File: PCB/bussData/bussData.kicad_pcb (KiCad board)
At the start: 2 copper layers, 104.1 x 57.2 mm, 13 parts, among them M3 MountingHole_3.2mm_M3

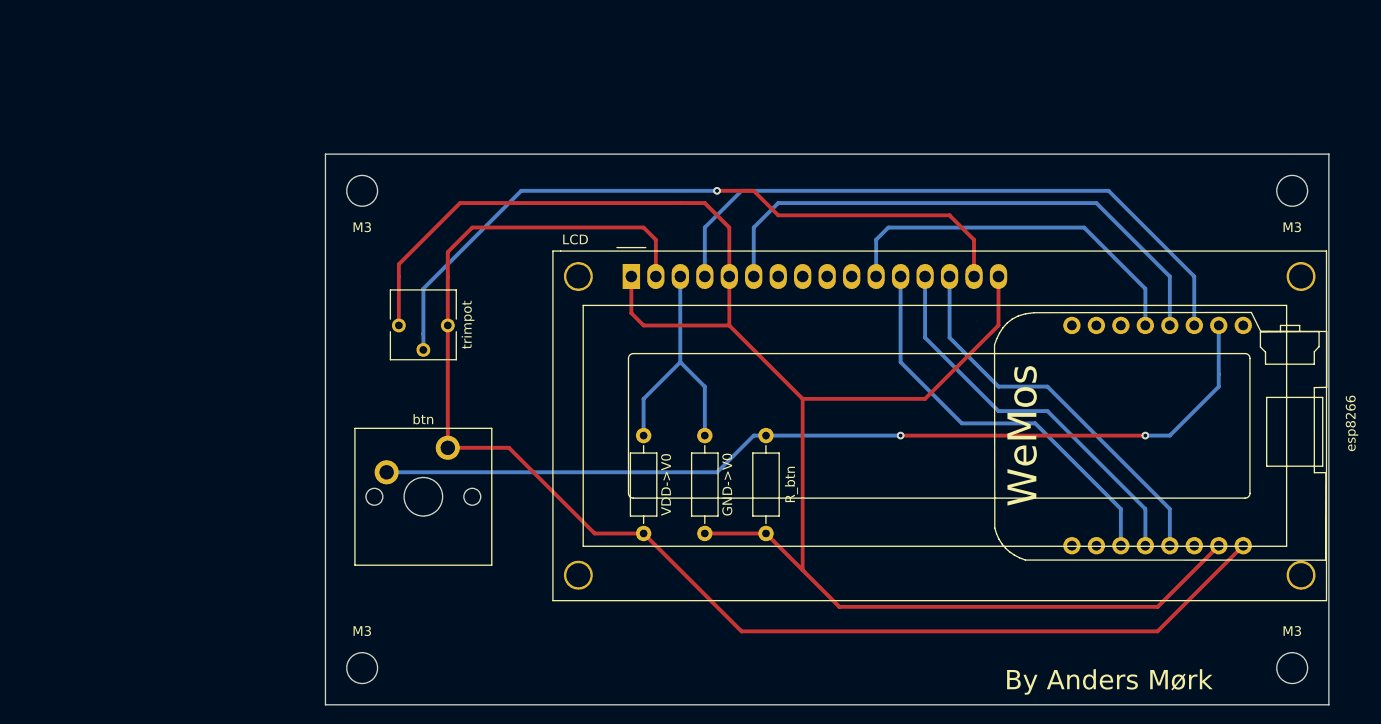
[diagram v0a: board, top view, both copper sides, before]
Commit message: updated pcb
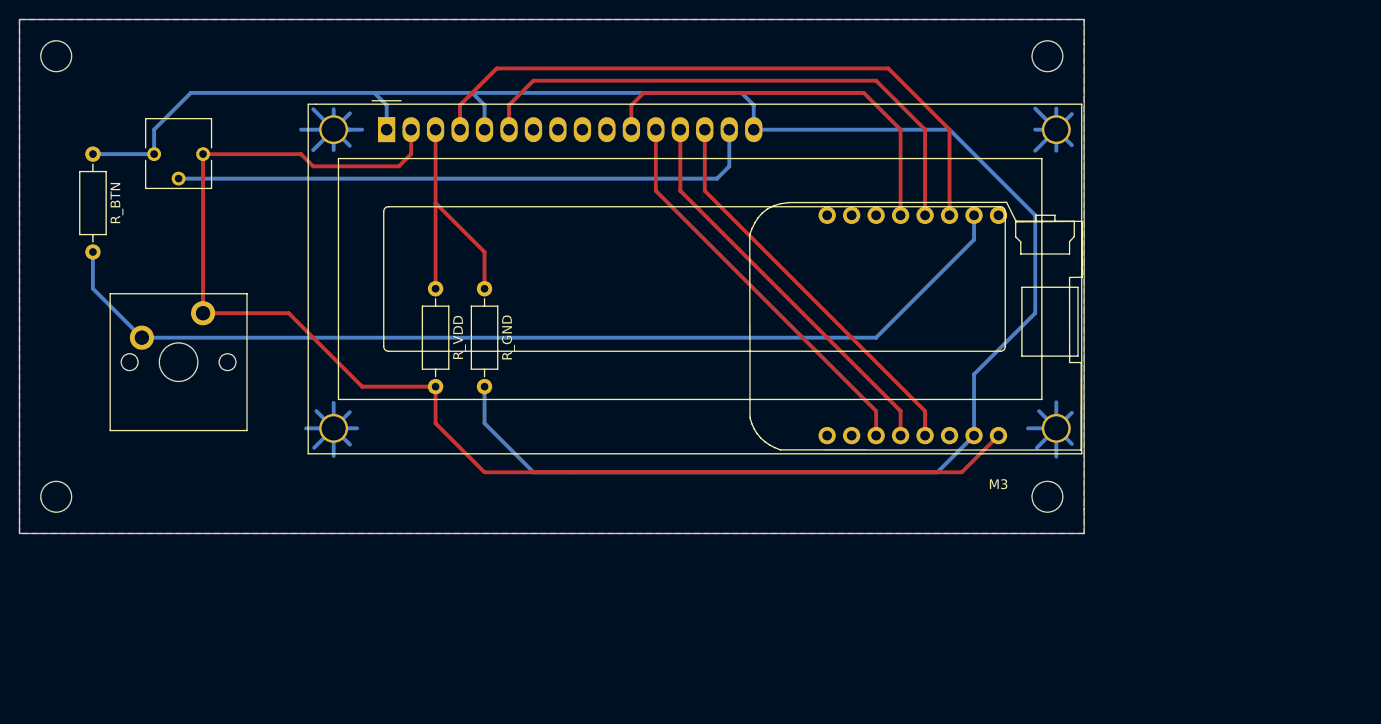
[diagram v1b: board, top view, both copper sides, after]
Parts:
- removed ? (x2): , 
- removed GND->V0, R_btn, VDD->V0: ?, Resistor_THT:R_Axial_DIN0207_L6.3mm_D2.5mm_P10.16mm_Horizontal
- removed LCD: RC1602A, Display:WC1602A
- removed the M3 at (209.6, 72.4)
- removed the M3 at (209.6, 121.9)
- removed the M3 at (113.0, 72.4)
- removed the M3 at (113.0, 121.9)
- removed btn: SW_Push_Open, Switch_Keyboard_Cherry_MX:SW_Cherry_MX_PCB_1.00u
- removed esp8266: WeMos_d1_mini, Module:D1_mini_board
- removed trimpot: R_POT_TRIM, Potentiometer_THT:Potentiometer_Vishay_T73YP_Vertical
- added DIM1: R_POT_TRIM, Potentiometer_THT:Potentiometer_Vishay_T73YP_Vertical, F.Cu at (91.4, 68.6)
- added LCD1: RC1602A, Display:WC1602A, F.Cu at (115.6, 66.0)
- added M3: MountingHole_3.2mm_M3, MountingHole:MountingHole_3.2mm_M3, F.Cu at (184.2, 104.1)
- added REF**: MountingHole_3.2mm_M3, MountingHole:MountingHole_3.2mm_M3, F.Cu at (81.3, 104.1)
- added REF**: MountingHole_3.2mm_M3, MountingHole:MountingHole_3.2mm_M3, F.Cu at (81.3, 58.4)
- added REF**: MountingHole_3.2mm_M3, MountingHole:MountingHole_3.2mm_M3, F.Cu at (184.2, 58.4)
- added R_BTN: ?, Resistor_THT:R_Axial_DIN0207_L6.3mm_D2.5mm_P10.16mm_Horizontal, F.Cu at (85.1, 68.6)
- added R_GND: ?, Resistor_THT:R_Axial_DIN0207_L6.3mm_D2.5mm_P10.16mm_Horizontal, F.Cu at (125.7, 82.5)
- added R_VDD: ?, Resistor_THT:R_Axial_DIN0207_L6.3mm_D2.5mm_P10.16mm_Horizontal, F.Cu at (120.7, 82.5)
- added btn1: SW_Push_Open, Switch_Keyboard_Cherry_MX:SW_Cherry_MX_PCB_1.00u, F.Cu at (94.0, 90.2)
- added esp8266 D1 Wemos mini: WeMos_mini, Module:D1_mini_board, F.Cu at (171.4, 86.4)
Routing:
- net (no net): track 0.00 -> 80.3 mm
- net Net-(DIM1-Pad1): track 185.2 -> 201.1 mm
- net Net-(DIM1-Pad2): track 73.6 -> 61.5 mm, vias 1 -> 0
- net Net-(R_btn1-Pad2): track 96.4 -> 104.1 mm, vias 2 -> 0
- net Net-(DIM1-Pad3): track 141.8 -> 134.9 mm
- net Net-(LCD1-Pad11): track 38.7 -> 41.5 mm
- net Net-(LCD1-Pad14): track 40.4 -> 41.2 mm
- net Net-(LCD1-Pad13): track 40.4 -> 41.2 mm
- net Net-(GND1-Pad1): track 26.8 -> 27.5 mm
- net Net-(LCD1-Pad12): track 41.9 -> 41.2 mm
- added copper zone on B.Cu, net Net-(DIM1-Pad1)
- added copper zone on F.Cu, net Net-(DIM1-Pad3)
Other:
- board size 104.1 x 57.2 mm -> 110.5 x 53.3 mm
